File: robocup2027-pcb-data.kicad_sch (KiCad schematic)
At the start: 7 parts, among them U1 ESP32-DEVKITC-32E

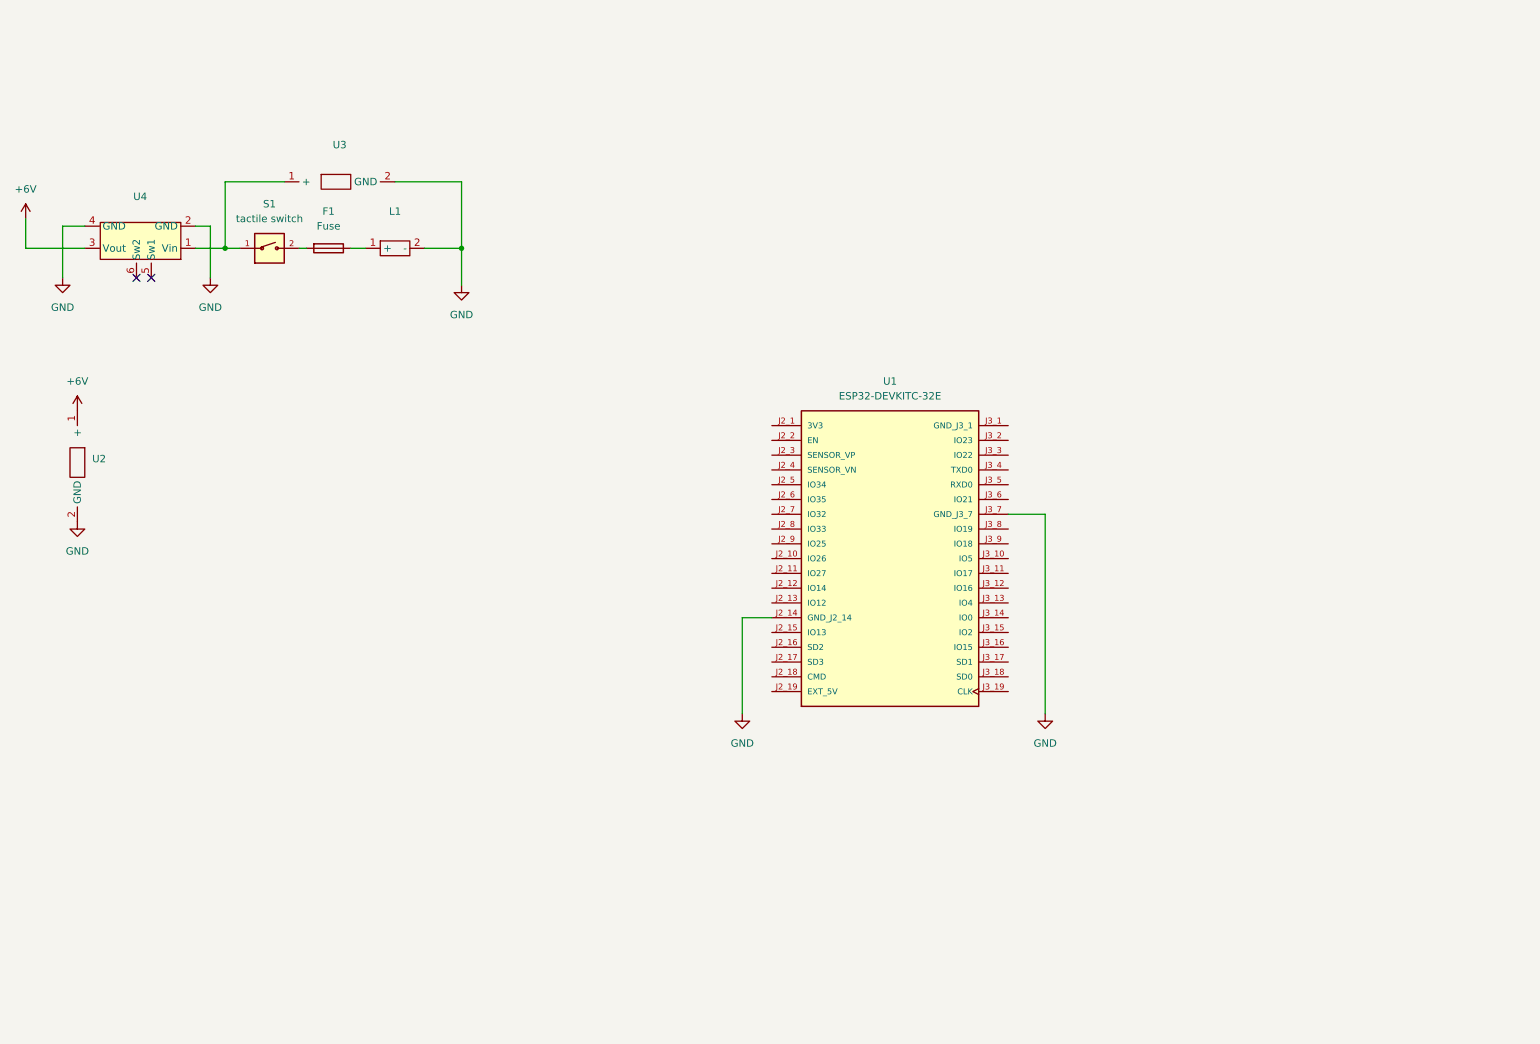
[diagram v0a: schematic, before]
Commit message: new data
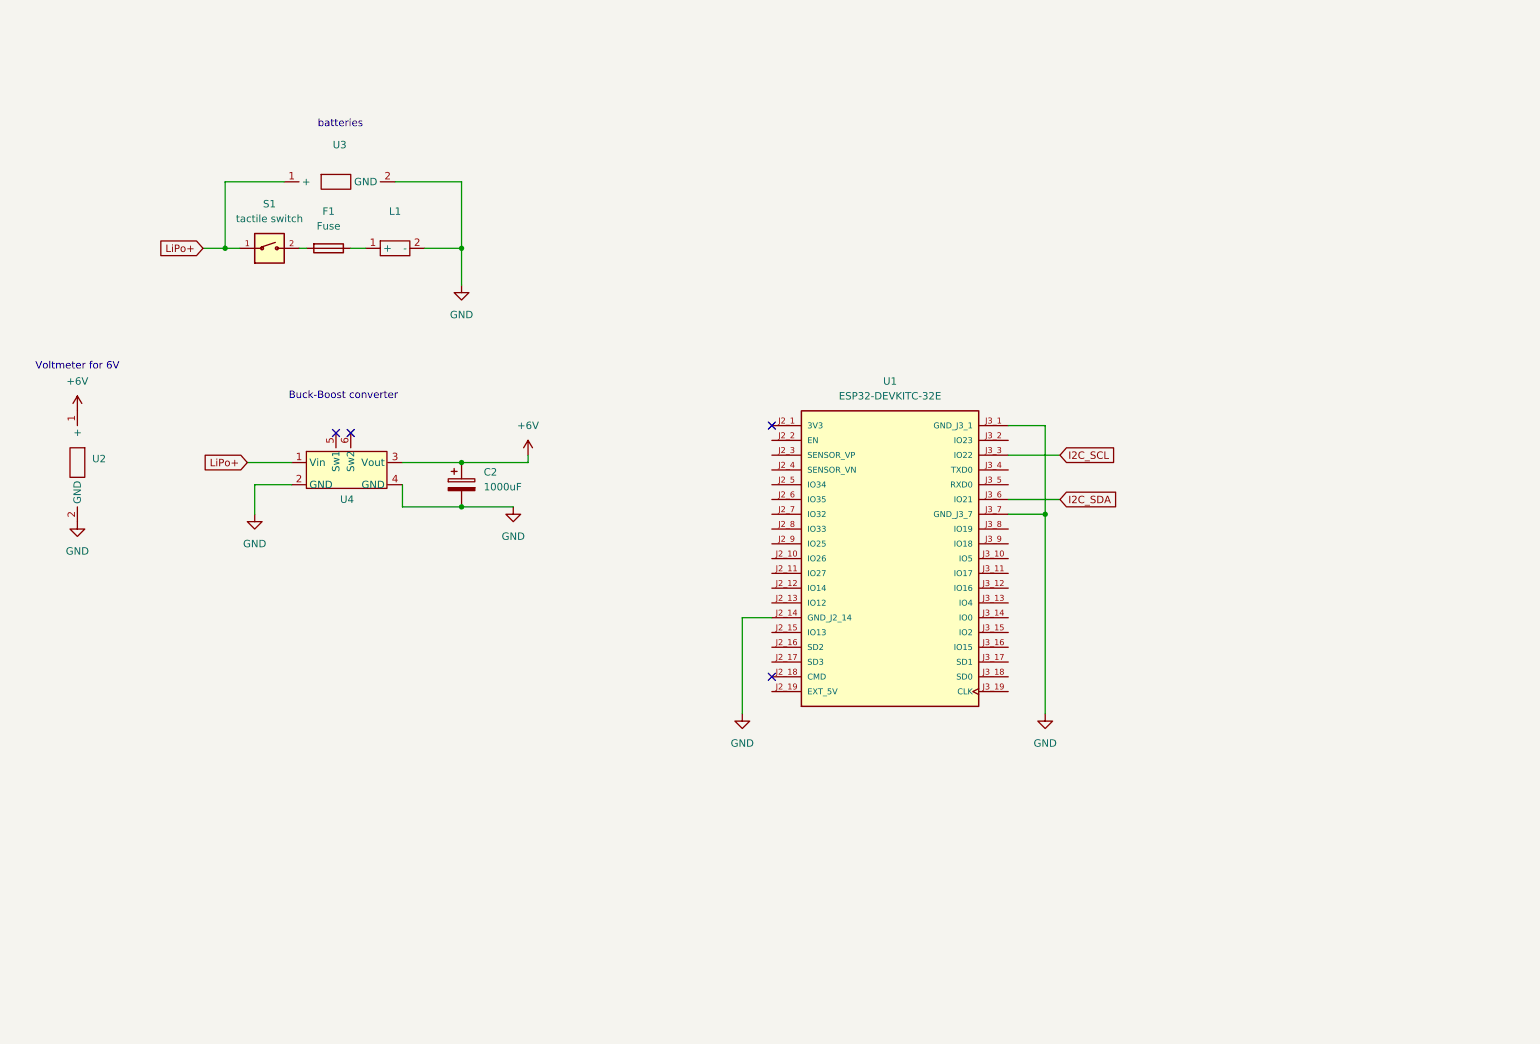
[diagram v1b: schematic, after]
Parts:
- added C2: 1000uF, symbol Device:C_Polarized
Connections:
- net +6V: now also C2.1
- net GND: now also U1.J3_1 (GND_J3_1), C2.2
- net LiPo+: now reaches S1.1, U3.1 (+), U4.1 (Vin)
- net I2C_SCL: now reaches U1.J3_3 (IO22)
- net I2C_SDA: now reaches U1.J3_6 (IO21)
- no-connect marks 2 -> 4
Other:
- note added: "Buck-Boost converter"
- note added: "Voltmeter for 6V"
- note added: "batteries"
- moved on the sheet: U4

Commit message: updating schematics
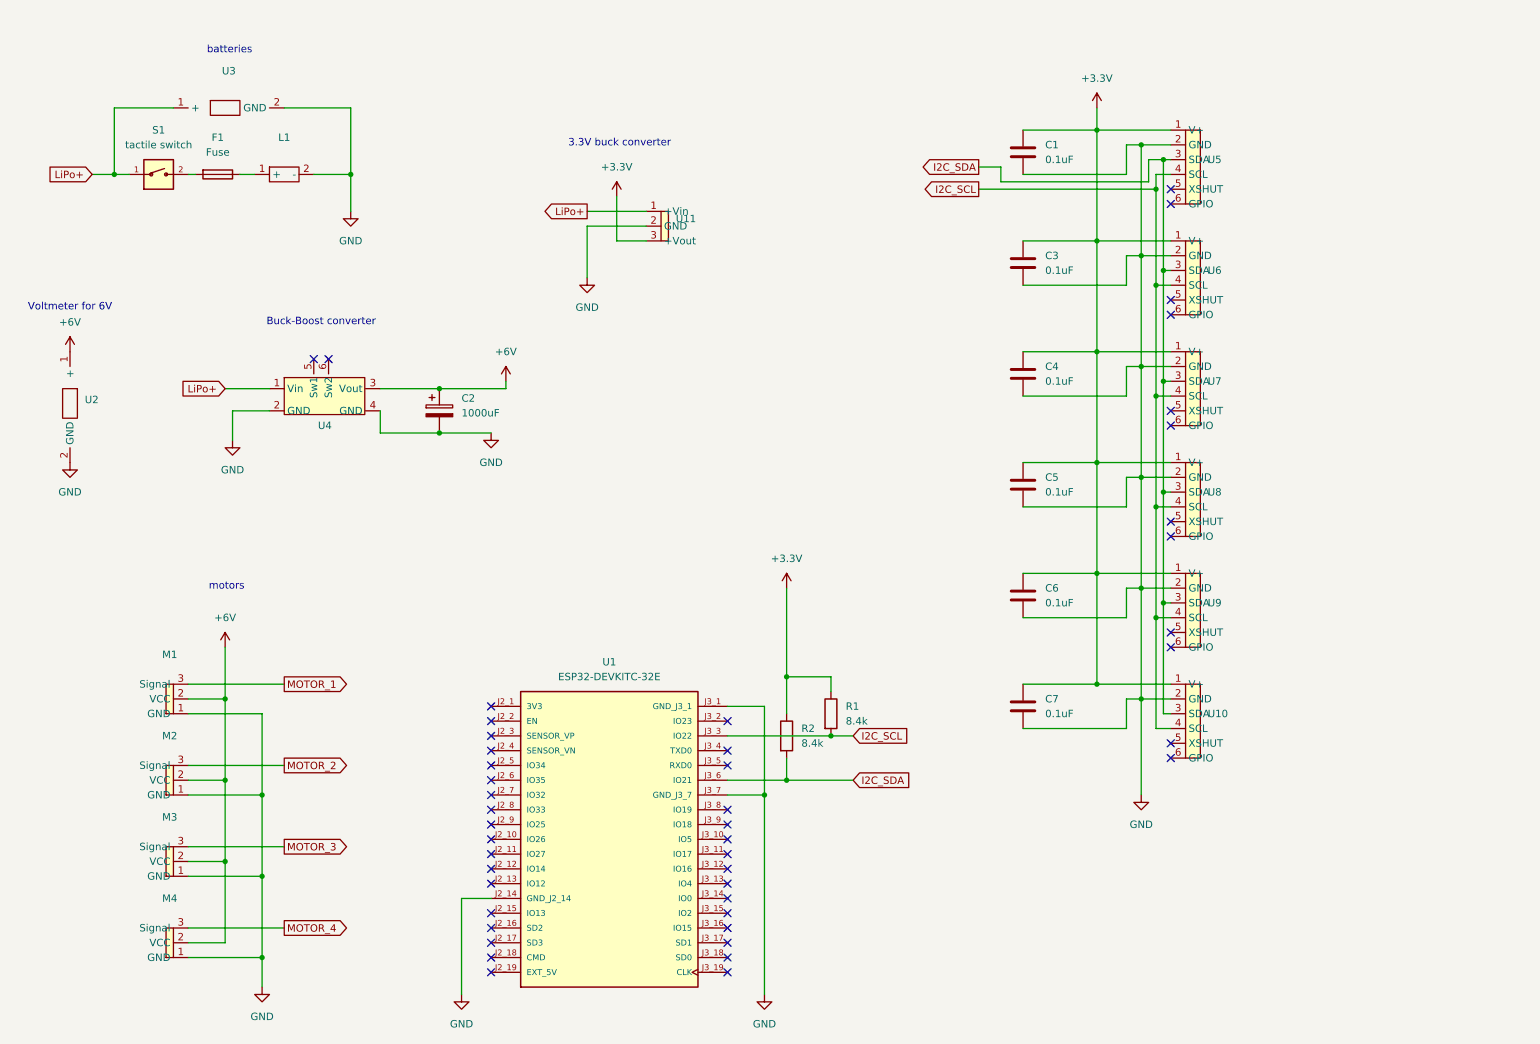
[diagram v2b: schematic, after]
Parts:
- added C1, C3, C4, C5, C6, C7: 0.1uF, symbol Device:C
- added M1, M2, M3, M4: ~, symbol robo:STS3032
- added R1, R2: 8.4k, symbol Device:R
- added U10, U5, U6, U7, U8, U9: ~, symbol robo:Tof-VL53L0X
- added U11: ~, symbol robo:DCDC-3.3v
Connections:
- net +6V: now also M1.2 (VCC), M2.2 (VCC), M3.2 (VCC), M4.2 (VCC)
- net GND: now also C1.2, C3.2, C4.2, C5.2, C6.2, C7.2, M1.1 (GND), M2.1 (GND), M3.1 (GND), M4.1 (GND), U10.2 (GND), U11.2 (GND), U5.2 (GND), U6.2 (GND), U7.2 (GND), U8.2 (GND), U9.2 (GND)
- net I2C_SCL: now also R1.2, U10.4 (SCL), U5.4 (SCL), U6.4 (SCL), U7.4 (SCL), U8.4 (SCL), U9.4 (SCL)
- net I2C_SDA: now also R2.2, U10.3 (SDA), U5.3 (SDA), U6.3 (SDA), U7.3 (SDA), U8.3 (SDA), U9.3 (SDA)
- net LiPo+: now also U11.1 (+Vin)
- new net +3.3V: C1.1, C3.1, C4.1, C5.1, C6.1, C7.1, R1.1, R2.1, U10.1 (V+), U11.3 (+Vout), U5.1 (V+), U6.1 (V+), U7.1 (V+), U8.1 (V+), U9.1 (V+)
- new net MOTOR_1: M1.3 (Signal)
- new net MOTOR_2: M2.3 (Signal)
- new net MOTOR_3: M3.3 (Signal)
- new net MOTOR_4: M4.3 (Signal)
- no-connect marks 4 -> 47
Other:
- note added: "3.3V buck converter"
- note added: "motors"
- moved on the sheet: C2, F1, L1, S1, U1, U2, U3, U4

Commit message: end of the day
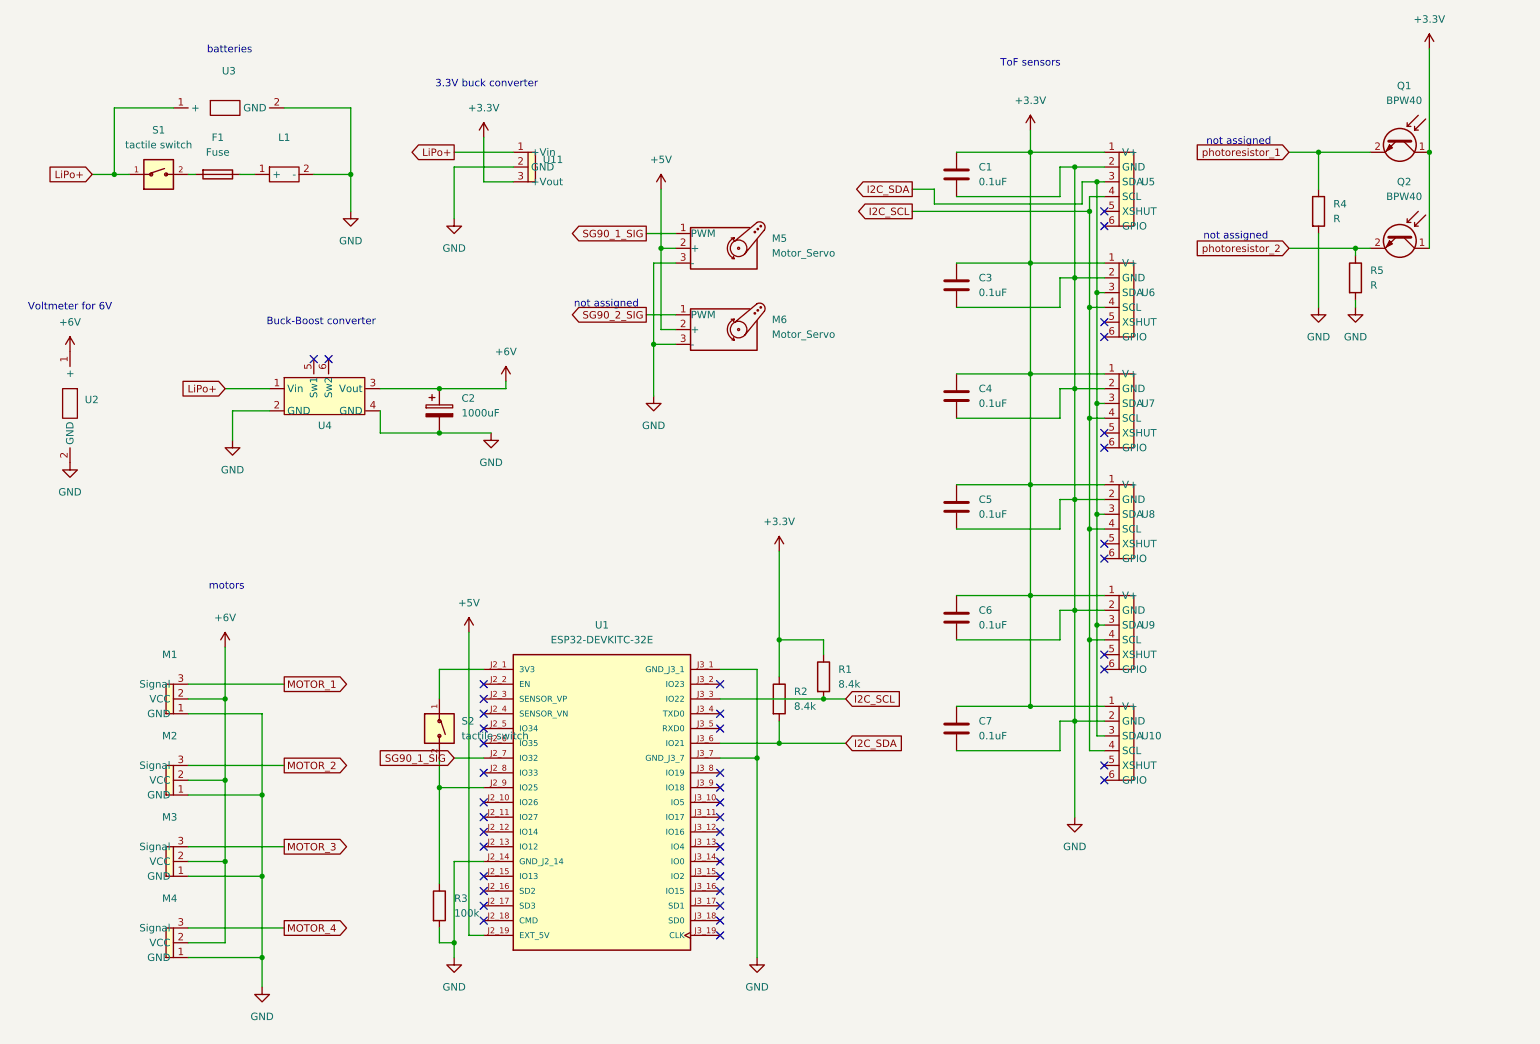
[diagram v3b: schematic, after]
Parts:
- added M5, M6: Motor_Servo, symbol Motor:Motor_Servo
- added Q1, Q2: BPW40, LED_THT:LED_D5.0mm_Clear, symbol Sensor_Optical:BPW40
- added R3: 100k, symbol Device:R
- added R4, R5: R, symbol Device:R
- added S2: tactile switch, 4-1437565-0:SW_4-1437565-0, symbol robo:tactile switch
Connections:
- net +3.3V: now also Q1.1 (C), Q2.1 (C)
- net GND: now also M5.3 (-), M6.3 (-), R3.2, R4.2, R5.2
- net at U1.J2_1 (3V3): now also S2.1
- net +5V: now reaches U1.J2_19 (EXT_5V)
- net +5V: now also M5.2 (+), M6.2 (+)
- net SG90_1_SIG: now reaches U1.J2_7 (IO32)
- net SG90_1_SIG: now also M5.1 (PWM)
- net at U1.J2_9 (IO25): now also R3.1, S2.2
- new net SG90_2_SIG: M6.1 (PWM)
- new net photoresistor_1: Q1.2 (E), R4.1
- new net photoresistor_2: Q2.2 (E), R5.1
- no-connect marks 47 -> 43
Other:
- note added: "ToF sensors"
- note added: "not assigned"
- moved on the sheet: C1, C3, C4, C5, C6, C7, R1, R2, U1, U10, U11, U5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

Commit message: end of the day
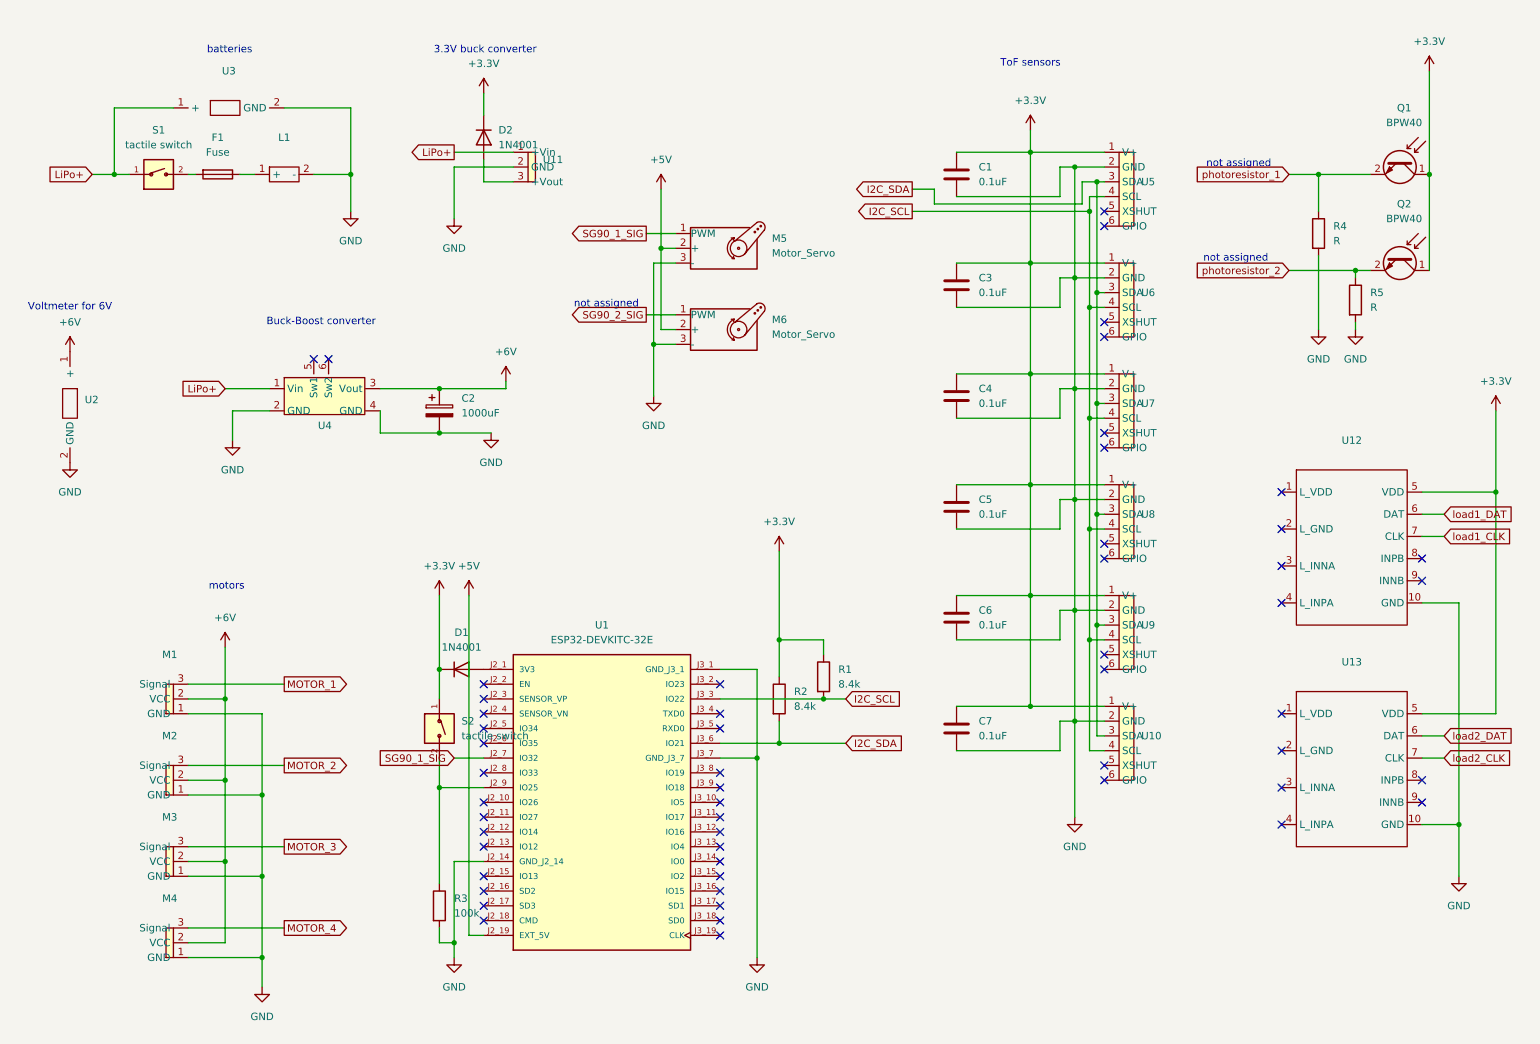
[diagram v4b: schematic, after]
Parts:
- added D1, D2: 1N4001, Diode_THT:D_DO-41_SOD81_P10.16mm_Horizontal, symbol Diode:1N4001
- added U12, U13: ~, symbol robo:AE-HX711-SIP
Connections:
- net +3.3V: now also S2.1, D1.1 (K), D2.1 (K), U12.5 (VDD), U13.5 (VDD); no longer U11.3 (+Vout)
- net GND: now also U12.10 (GND), U13.10 (GND)
- net at U1.J2_1 (3V3): now also D1.2 (A); no longer S2.1
- new net: D2.2 (A), U11.3 (+Vout)
- new net load1_CLK: U12.7 (CLK)
- new net load1_DAT: U12.6 (DAT)
- new net load2_CLK: U13.7 (CLK)
- new net load2_DAT: U13.6 (DAT)
- no-connect marks 43 -> 55
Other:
- moved on the sheet: Q1, Q2, R4, R5
